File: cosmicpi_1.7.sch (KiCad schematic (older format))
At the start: 102 parts, among them J1 Barrel_Jack_Switch, J2 SMA, J3 USB_B_Micro, J6 SWD, J7 Raspberry_Pi_2_3, U1 MCP47CMB22, U10 TPS62163DSG, U11 LM555, U12 LM555, U16 LP2985-3.3, U2 STM32F401RETx, U3 L76-M33, U4 74HC00, U5 BME280, U6 LM555, U7 LSM9DS1, U8 ESP-12F, U9 MAX991, Y1 8 MHz, Y2 32.768KHz

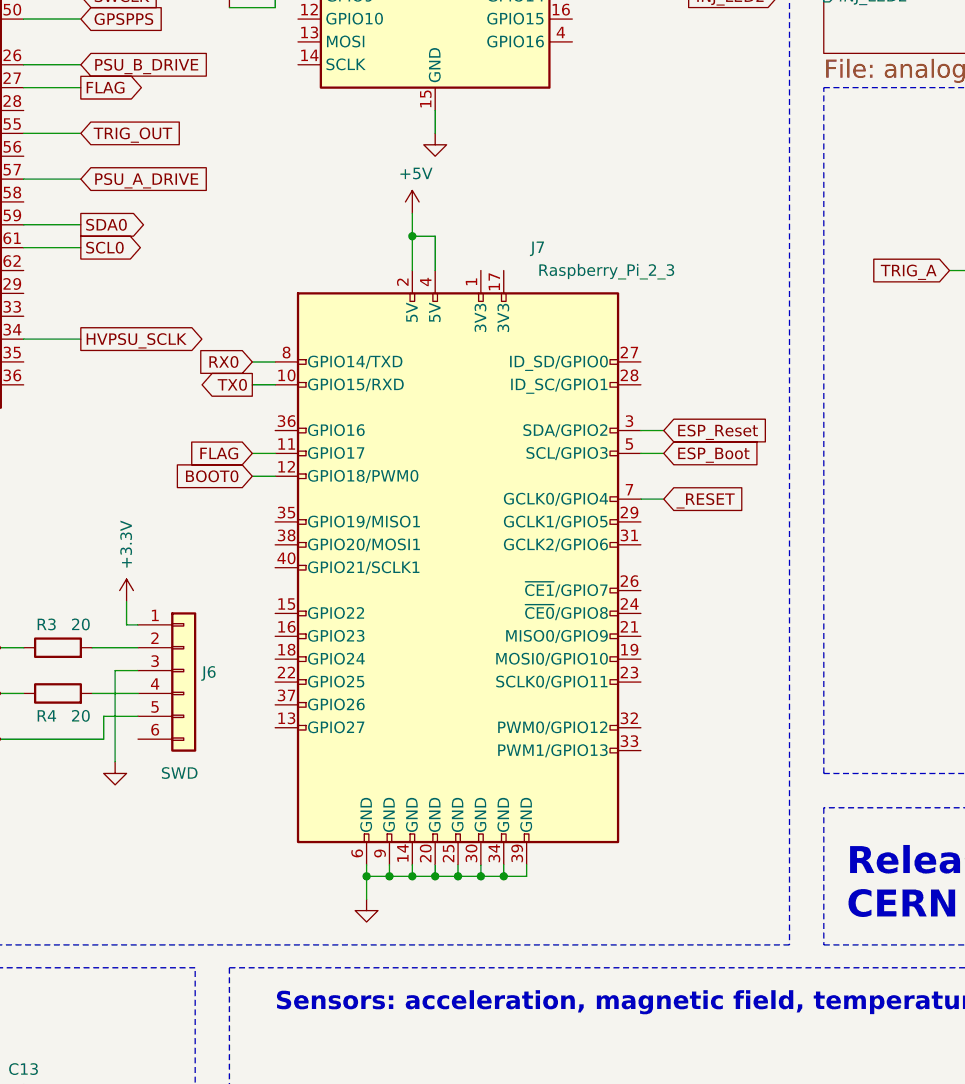
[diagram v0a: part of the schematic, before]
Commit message: updated a little
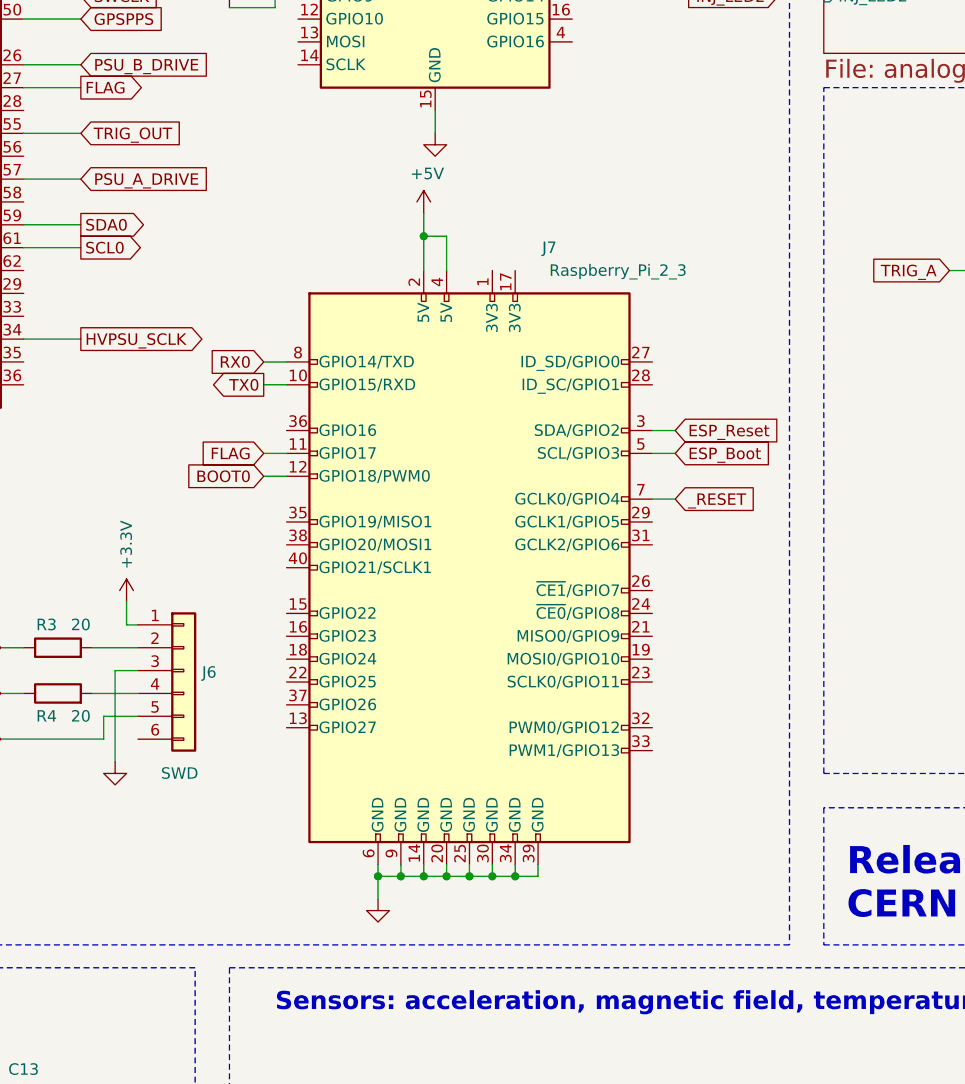
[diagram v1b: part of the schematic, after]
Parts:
- D10, D9: footprint (none) -> Diode_SMD:D_SMA
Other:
- moved on the sheet: J7
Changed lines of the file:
@@
 L Connector:Raspberry_Pi_2_3 J7
 U 1 1 5C85EEA0
-P 5300 5900
-F 0 "J7" H 5650 7300 50  0000 C CNN
-F 1 "Raspberry_Pi_2_3" H 5950 7200 50  0000 C CNN
-F 2 "Connector_PinSocket_2.54mm:PinSocket_2x20_P2.54mm_Vertical_SMD" H 5300 5900 50  0001 C CNN
-F 3 "https://www.raspberrypi.org/documentation/hardware/raspberrypi/schematics/rpi_SCH_3bplus_1p0_reduced.pdf" H 5300 5900 50  0001 C CNN
-	1    5300 5900
+P 5350 5900
+F 0 "J7" H 5700 7300 50  0000 C CNN
+F 1 "Raspberry_Pi_2_3" H 6000 7200 50  0000 C CNN
+F 2 "Connector_PinSocket_2.54mm:PinSocket_2x20_P2.54mm_Vertical_SMD" H 5350 5900 50  0001 C CNN
+F 3 "https://www.raspberrypi.org/documentation/hardware/raspberrypi/schematics/rpi_SCH_3bplus_1p0_reduced.pdf" H 5350 5900 50  0001 C CNN
+	1    5350 5900
 	1    0    0    -1
 $EndComp
@@
 L power:GND #PWR046
 U 1 1 5C8DAC28
-P 4900 7350
-F 0 "#PWR046" H 4900 7100 50  0001 C CNN
-F 1 "GND" H 4905 7177 50  0001 C CNN
-F 2 "" H 4900 7350 50  0001 C CNN
-F 3 "" H 4900 7350 50  0001 C CNN
-	1    4900 7350
-	1    0    0    -1
-$EndComp
-Wire Wire Line
-	4900 7200 4900 7250
-Wire Wire Line
-	4900 7250 5000 7250
-Wire Wire Line
-	5600 7250 5600 7200
-Connection ~ 4900 7250
-Wire Wire Line
-	4900 7250 4900 7350
-Wire Wire Line
-	5000 7200 5000 7250
-Connection ~ 5000 7250
-Wire Wire Line
-	5000 7250 5100 7250
-Wire Wire Line
-	5100 7200 5100 7250
-Connection ~ 5100 7250
-Wire Wire Line
-	5100 7250 5200 7250
-Wire Wire Line
-	5200 7200 5200 7250
-Connection ~ 5200 7250
-Wire Wire Line
-	5200 7250 5300 7250
-Wire Wire Line
-	5300 7200 5300 7250
-Connection ~ 5300 7250
-Wire Wire Line
-	5300 7250 5400 7250
-Wire Wire Line
-	5400 7200 5400 7250
-Connection ~ 5400 7250
-Wire Wire Line
-	5400 7250 5500 7250
-Wire Wire Line
-	5500 7200 5500 7250
-Connection ~ 5500 7250
-Wire Wire Line
-	5500 7250 5600 7250
+P 4950 7350
+F 0 "#PWR046" H 4950 7100 50  0001 C CNN
+F 1 "GND" H 4955 7177 50  0001 C CNN
+F 2 "" H 4950 7350 50  0001 C CNN
+F 3 "" H 4950 7350 50  0001 C CNN
+	1    4950 7350
+	1    0    0    -1
+$EndComp
+Wire Wire Line
+	4950 7200 4950 7250
+Wire Wire Line
+	4950 7250 5050 7250
+Wire Wire Line
+	5650 7250 5650 7200
+Connection ~ 4950 7250
+Wire Wire Line
+	4950 7250 4950 7350
+Wire Wire Line
+	5050 7200 5050 7250
+Connection ~ 5050 7250
+Wire Wire Line
+	5050 7250 5150 7250
+Wire Wire Line
+	5150 7200 5150 7250
+Connection ~ 5150 7250
+Wire Wire Line
+	5150 7250 5250 7250
+Wire Wire Line
+	5250 7200 5250 7250
+Connection ~ 5250 7250
+Wire Wire Line
+	5250 7250 5350 7250
+Wire Wire Line
+	5350 7200 5350 7250
+Connection ~ 5350 7250
+Wire Wire Line
+	5350 7250 5450 7250
+Wire Wire Line
+	5450 7200 5450 7250
+Connection ~ 5450 7250
+Wire Wire Line
+	5450 7250 5550 7250
+Wire Wire Line
+	5550 7200 5550 7250
+Connection ~ 5550 7250
+Wire Wire Line
+	5550 7250 5650 7250
 Wire Wire Line
 	3400 2300 3700 2300
@@
 L power:+5V #PWR047
 U 1 1 5CA23FDD
-P 5100 4350
-F 0 "#PWR047" H 5100 4200 50  0001 C CNN
-F 1 "+5V" H 5115 4523 50  0000 C CNN
-F 2 "" H 5100 4350 50  0001 C CNN
-F 3 "" H 5100 4350 50  0001 C CNN
-	1    5100 4350
-	1    0    0    -1
-$EndComp
-Wire Wire Line
-	5100 4350 5100 4450
-Wire Wire Line
-	5100 4450 5200 4450
-Wire Wire Line
-	5200 4450 5200 4600
-Connection ~ 5100 4450
-Wire Wire Line
-	5100 4450 5100 4600
-Text GLabel 4400 5100 0    50   Output ~ 0
+P 5150 4350
+F 0 "#PWR047" H 5150 4200 50  0001 C CNN
+F 1 "+5V" H 5165 4523 50  0000 C CNN
+F 2 "" H 5150 4350 50  0001 C CNN
+F 3 "" H 5150 4350 50  0001 C CNN
+	1    5150 4350
+	1    0    0    -1
+$EndComp
+Wire Wire Line
+	5150 4350 5150 4450
+Wire Wire Line
+	5150 4450 5250 4450
+Wire Wire Line
+	5250 4450 5250 4600
+Connection ~ 5150 4450
+Wire Wire Line
+	5150 4450 5150 4600
+Text GLabel 4450 5100 0    50   Output ~ 0
 TX0
-Text GLabel 4400 5000 0    50   Input ~ 0
+Text GLabel 4450 5000 0    50   Input ~ 0
 RX0
 Wire Wire Line
-	4400 5000 4500 5000
-Wire Wire Line
-	4400 5100 4500 5100
-Text GLabel 4400 5400 0    50   Input ~ 0
+	4450 5000 4550 5000
+Wire Wire Line
+	4450 5100 4550 5100
+Text GLabel 4450 5400 0    50   Input ~ 0
 FLAG
-Text GLabel 4400 5500 0    50   Input ~ 0
+Text GLabel 4450 5500 0    50   Input ~ 0
 BOOT0
 Wire Wire Line
-	4400 5400 4500 5400
-Wire Wire Line
-	4500 5500 4400 5500
-Text GLabel 6200 5600 2    50   Input ~ 0
+	4450 5400 4550 5400
+Wire Wire Line
+	4550 5500 4450 5500
+Text GLabel 6250 5600 2    50   Input ~ 0
 _RESET
 Wire Wire Line
-	6100 5600 6200 5600
+	6150 5600 6250 5600
 $Comp
 L Connector:USB_B_Micro J3
@@
 F 0 "D9" H 11550 8065 50  0000 C CNN
 F 1 "B140" H 11550 7974 50  0000 C CNN
-F 2 "" H 11550 7800 50  0001 C CNN
+F 2 "Diode_SMD:D_SMA" H 11550 7800 50  0001 C CNN
 F 3 "~" H 11550 7800 50  0001 C CNN
 	1    11550 7800
@@
 F 0 "D10" H 2450 7015 50  0000 C CNN
 F 1 "B140" H 2450 6924 50  0000 C CNN
-F 2 "" H 2450 6750 50  0001 C CNN
+F 2 "Diode_SMD:D_SMA" H 2450 6750 50  0001 C CNN
 F 3 "~" H 2450 6750 50  0001 C CNN
 	1    2450 6750
@@
 Wire Wire Line
 	5900 2900 5800 2900
-Text GLabel 6200 5300 2    50   Input ~ 0
+Text GLabel 6250 5300 2    50   Input ~ 0
 ESP_Reset
-Text GLabel 6200 5400 2    50   Input ~ 0
+Text GLabel 6250 5400 2    50   Input ~ 0
 ESP_Boot
 Wire Wire Line
-	6100 5300 6200 5300
-Wire Wire Line
-	6100 5400 6200 5400
+	6150 5300 6250 5300
+Wire Wire Line
+	6150 5400 6250 5400
 $Comp
 L Device:R R71
